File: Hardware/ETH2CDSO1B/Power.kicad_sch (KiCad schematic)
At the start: 13 parts, among them U602 LM317L_SOT-89, U906 LM1117SX-5.0/NOPB, U908 LM2990SX-5.0

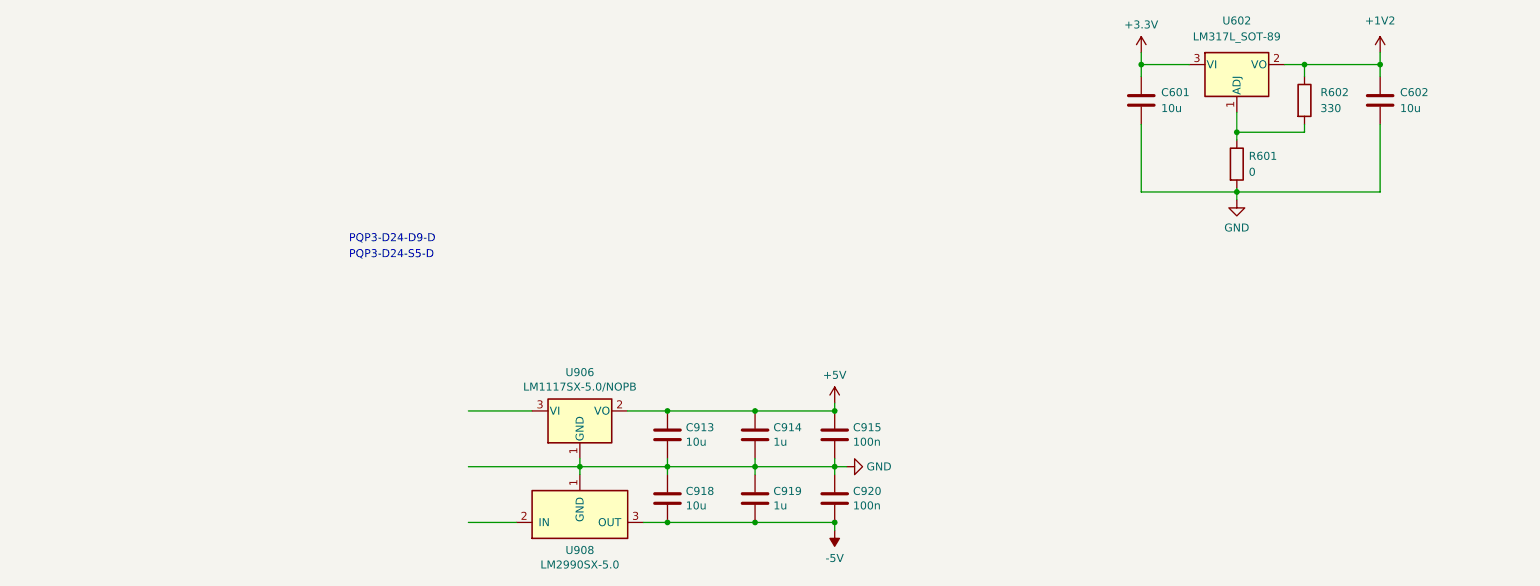
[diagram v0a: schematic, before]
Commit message: Hardware
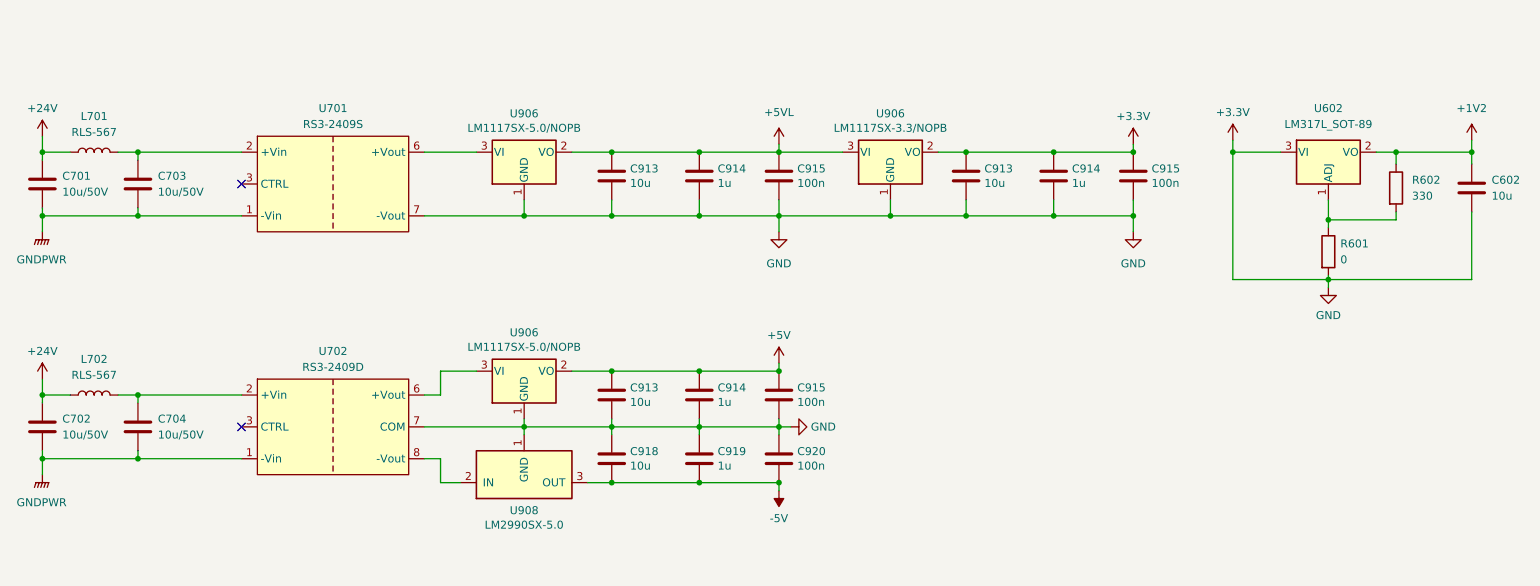
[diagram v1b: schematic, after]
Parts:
- removed C601: 10u, symbol Device:C
- added C701, C702, C703, C704: 10u/50V, Capacitor_SMD:C_1206_3216Metric_Pad1.33x1.80mm_HandSolder, symbol Device:C
- added C913 (x2): 10u, Capacitor_SMD:C_1206_3216Metric_Pad1.33x1.80mm_HandSolder, symbol Device:C
- added C914 (x2): 1u, Capacitor_SMD:C_1206_3216Metric_Pad1.33x1.80mm_HandSolder, symbol Device:C
- added C915 (x2): 100n, Capacitor_SMD:C_1206_3216Metric_Pad1.33x1.80mm_HandSolder, symbol Device:C
- added L701, L702: RLS-567, symbol Device:L
- added U701: RS3-2409S, ETH2CDSO1B:RS3-xxxxD, symbol ETH2CDSO1B:RS3-xxxxS
- added U702: RS3-2409D, ETH2CDSO1B:RS3-xxxxD, symbol ETH2CDSO1B:RS3-xxxxD
- added U906: LM1117SX-5.0/NOPB, Package_TO_SOT_SMD:TO-263-3_TabPin2, symbol Regulator_Linear:TLV1117-50
- added U906: LM1117SX-3.3/NOPB, Package_TO_SOT_SMD:TO-263-3_TabPin2, symbol Regulator_Linear:TLV1117-50
- R601, R602: footprint (none) -> Resistor_SMD:R_0603_1608Metric_Pad0.98x0.95mm_HandSolder
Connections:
- net GND is gone; now on net +3.3V: C602.2, C913.2, C914.2, C915.2, C918.1, C919.1, C920.1, R601.2, U906.1 (GND), U908.1 (GND)
- net +3.3V: now also C913.1, C913.2, C913.2, C914.1, C914.2, C914.2, C915.1, C915.2, C915.2, U701.7 (-Vout), U702.7 (COM), U906.1 (GND), U906.1 (GND), U906.2 (VO)
- net at U908.2 (IN): now also U702.8 (-Vout)
- net at U906.3 (VI): now also U702.6 (+Vout)
- new net: C704.1, L702.2, U702.2 (+Vin)
- new net: U701.6 (+Vout), U906.3 (VI)
- new net: C703.1, L701.2, U701.2 (+Vin)
- new net +24V: C701.1, C702.1, L701.1, L702.1
- new net +5VL: C913.1, C914.1, C915.1, U906.2 (VO), U906.3 (VI)
- new net GNDPWR: C701.2, C702.2, C703.2, C704.2, U701.1 (-Vin), U702.1 (-Vin)
- no-connect marks 0 -> 2
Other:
- note removed: "PQP3-D24-D9-D"
- note removed: "PQP3-D24-S5-D"
- moved on the sheet: C602, C913, C914, C915, C918, C919, C920, R601, R602, U602, U906, U908
